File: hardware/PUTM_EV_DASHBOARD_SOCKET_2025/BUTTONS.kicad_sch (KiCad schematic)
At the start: 10 parts, among them SW1 SW_Push, SW2 SW_Push, SW3 SW_Push, SW4 SW_Push, SW5 SW_Push

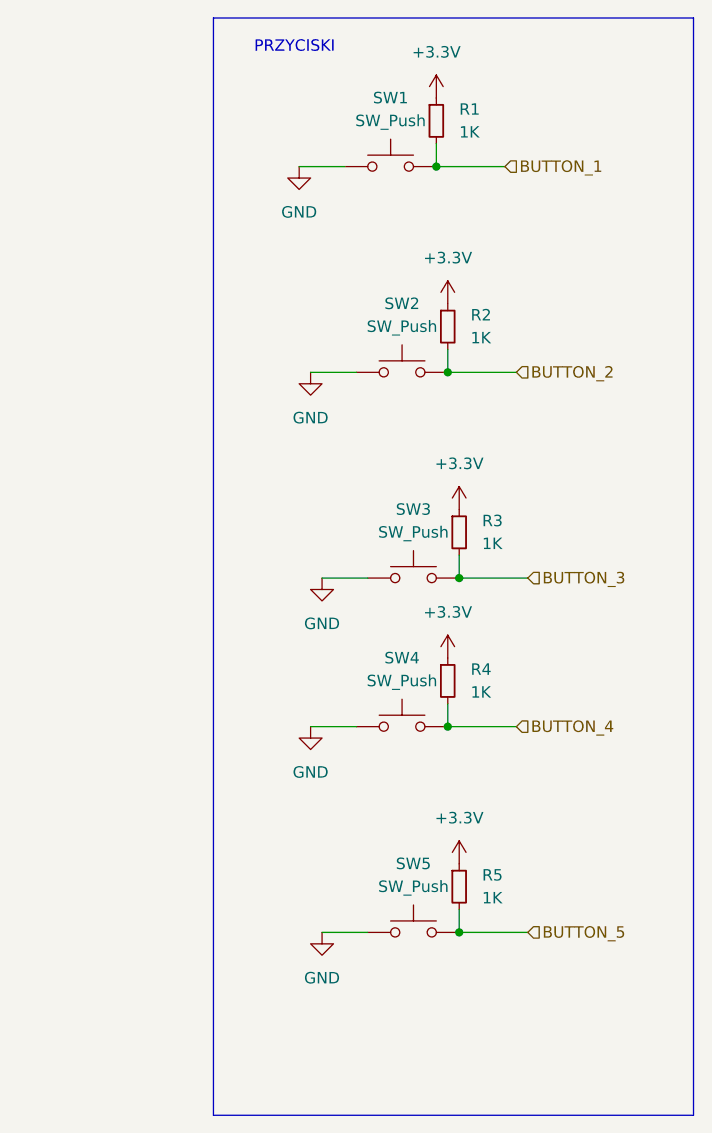
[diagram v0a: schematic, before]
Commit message: fixed layout
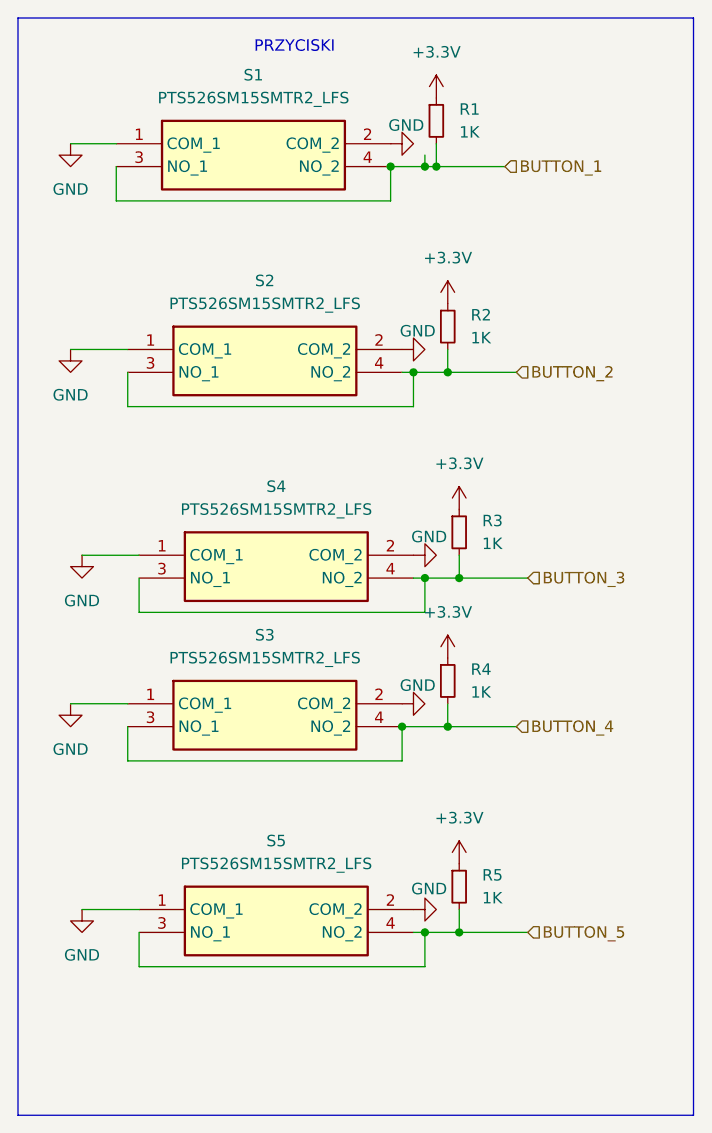
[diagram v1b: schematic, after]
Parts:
- removed SW1, SW2, SW3, SW4, SW5: SW_Push, Button_Switch_SMD:SW_Push_1P1T_NO_E-Switch_TL3301NxxxxxG, symbol Switch:SW_Push
- added S1, S2, S3, S4, S5: PTS526SM15SMTR2_LFS, PTS526SM15SMTR2LFS, symbol SamacSys_Parts:PTS526SM15SMTR2_LFS
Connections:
- net BUTTON_1: now also S1.3 (NO_1), S1.4 (NO_2)
- net BUTTON_2: now also S2.3 (NO_1), S2.4 (NO_2)
- net BUTTON_3: now also S4.3 (NO_1), S4.4 (NO_2)
- net BUTTON_4: now also S3.3 (NO_1), S3.4 (NO_2)
- net BUTTON_5: now also S5.3 (NO_1), S5.4 (NO_2)
- net GND: now also S1.1 (COM_1), S1.2 (COM_2), S2.1 (COM_1), S2.2 (COM_2), S3.1 (COM_1), S3.2 (COM_2), S4.1 (COM_1), S4.2 (COM_2), S5.1 (COM_1), S5.2 (COM_2)
